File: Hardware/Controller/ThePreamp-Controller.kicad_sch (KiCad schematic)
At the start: 23 parts, among them J1 8V, J2 Power relay trigger, J3 SPI DISPLAY 1, J4 SPI DISPLAY 2, J5 Digital Out, J6 3.3V (Opt), J7 Conn_01x03_Pin, J8 12V, SW1 RotaryEncoder_Switch, SW2 RotaryEncoder_Switch, U1 TSOP34838, U2 CAT24C64WI-GT3, U3 ESP32-DEVKIT-V1, U4 APC-817B1-SL

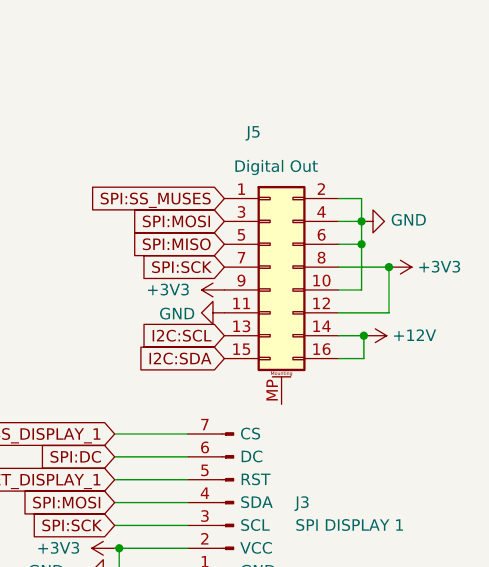
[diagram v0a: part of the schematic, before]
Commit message: Chassis placement new draft
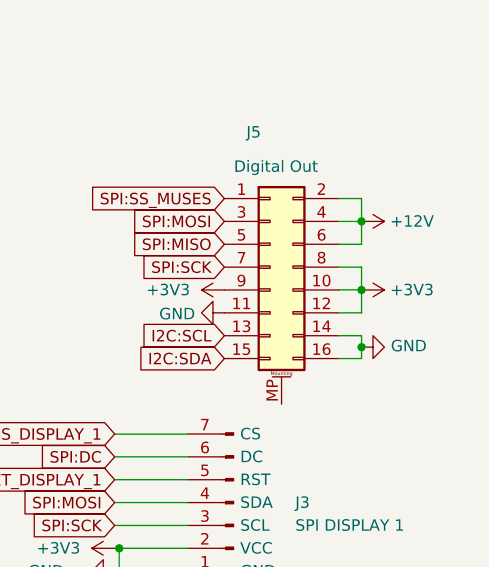
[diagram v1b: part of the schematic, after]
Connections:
- net +12V: now also J5.2 (Pin_2), J5.4 (Pin_4), J5.6 (Pin_6); no longer J5.14 (Pin_14), J5.16 (Pin_16)
- net +3V3: now also J5.10 (Pin_10)
- net GND: now also J5.14 (Pin_14), J5.16 (Pin_16); no longer J5.10 (Pin_10), J5.2 (Pin_2), J5.4 (Pin_4), J5.6 (Pin_6)
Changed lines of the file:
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@@
 	)
 	(junction
-		(at 263.906 62.484)
+		(at 263.906 73.914)
+		(diameter 0)
+		(color 0 0 0 0)
+	)
+	(junction
+		(at 263.906 59.944)
 		(diameter 0)
 		(color 0 0 0 0)
@@
 	)
 	(junction
-		(at 266.954 65.024)
+		(at 263.906 67.564)
 		(diameter 0)
 		(color 0 0 0 0)
@@
 	)
 	(junction
-		(at 264.16 72.644)
-		(diameter 0)
-		(color 0 0 0 0)
-	)
-	(junction
 		(at 117.856 153.67)
 		(diameter 0)
@@
 	)
 	(junction
-		(at 263.906 59.944)
-		(diameter 0)
-		(color 0 0 0 0)
-	)
-	(junction
 		(at 120.396 156.21)
 		(diameter 0)
@@
 	(wire
 		(pts
+			(xy 263.906 65.024) (xy 263.906 67.564)
+		)
+		(stroke
+			(width 0)
+			(type default)
+		)
+	)
+	(wire
+		(pts
+			(xy 263.906 62.484) (xy 263.906 59.944)
+		)
+		(stroke
+			(width 0)
+			(type default)
+		)
+	)
+	(wire
+		(pts
 			(xy 69.596 67.056) (xy 71.882 67.056)
 		)
@@
 	(wire
 		(pts
-			(xy 154.94 66.04) (xy 167.64 66.04)
+			(xy 263.906 57.404) (xy 263.906 59.944)
 		)
 		(stroke
@@
 	(wire
 		(pts
-			(xy 165.1 63.5) (xy 167.64 63.5)
+			(xy 154.94 66.04) (xy 167.64 66.04)
 		)
 		(stroke
@@
 	(wire
 		(pts
-			(xy 124.46 158.75) (xy 117.856 158.75)
+			(xy 165.1 63.5) (xy 167.64 63.5)
 		)
 		(stroke
@@
 	(wire
 		(pts
-			(xy 261.366 72.644) (xy 264.16 72.644)
+			(xy 124.46 158.75) (xy 117.856 158.75)
 		)
 		(stroke
@@
 	(wire
 		(pts
-			(xy 263.906 57.404) (xy 263.906 59.944)
+			(xy 261.366 75.184) (xy 263.906 75.184)
 		)
 		(stroke
@@
 	(wire
 		(pts
-			(xy 263.906 62.484) (xy 263.906 67.564)
+			(xy 263.906 67.564) (xy 263.906 70.104)
 		)
 		(stroke
@@
 	(wire
 		(pts
-			(xy 264.16 75.184) (xy 264.16 72.644)
-		)
-		(stroke
-			(width 0)
-			(type default)
-		)
-	)
-	(wire
-		(pts
 			(xy 236.474 93.726) (xy 244.602 93.726)
 		)
@@
 	(wire
 		(pts
-			(xy 261.366 75.184) (xy 264.16 75.184)
+			(xy 155.702 32.766) (xy 159.766 32.766)
 		)
 		(stroke
@@
 	(wire
 		(pts
-			(xy 155.702 32.766) (xy 159.766 32.766)
+			(xy 236.474 96.266) (xy 236.982 96.266)
 		)
 		(stroke
@@
 	(wire
 		(pts
-			(xy 236.474 96.266) (xy 236.982 96.266)
+			(xy 263.906 72.644) (xy 263.906 73.914)
 		)
 		(stroke
@@
 	(wire
 		(pts
-			(xy 261.366 70.104) (xy 266.954 70.104)
+			(xy 261.366 70.104) (xy 263.906 70.104)
 		)
 		(stroke
@@
 	(wire
 		(pts
-			(xy 263.906 59.944) (xy 263.906 62.484)
+			(xy 125.73 145.542) (xy 125.73 150.114)
 		)
 		(stroke
@@
 	(wire
 		(pts
-			(xy 125.73 145.542) (xy 125.73 150.114)
+			(xy 45.212 100.076) (xy 45.72 100.076)
 		)
 		(stroke
@@
 	(wire
 		(pts
-			(xy 45.212 100.076) (xy 45.72 100.076)
+			(xy 236.728 127.508) (xy 244.856 127.508)
 		)
 		(stroke
@@
 	(wire
 		(pts
-			(xy 236.728 127.508) (xy 244.856 127.508)
+			(xy 261.366 62.484) (xy 263.906 62.484)
 		)
 		(stroke
@@
 	(wire
 		(pts
-			(xy 261.366 62.484) (xy 263.906 62.484)
+			(xy 236.982 107.696) (xy 236.982 118.11)
 		)
 		(stroke
@@
 	(wire
 		(pts
-			(xy 236.982 107.696) (xy 236.982 118.11)
+			(xy 88.9 125.222) (xy 90.17 125.222)
 		)
 		(stroke
@@
 	(wire
 		(pts
-			(xy 88.9 125.222) (xy 90.17 125.222)
+			(xy 77.216 153.67) (xy 77.216 156.21)
 		)
 		(stroke
@@
 	(wire
 		(pts
-			(xy 77.216 153.67) (xy 77.216 156.21)
+			(xy 263.906 73.914) (xy 263.906 75.184)
 		)
 		(stroke
@@
 	(wire
 		(pts
-			(xy 266.954 65.024) (xy 266.954 70.104)
-		)
-		(stroke
-			(width 0)
-			(type default)
-		)
-	)
-	(wire
-		(pts
 			(xy 124.46 156.21) (xy 120.396 156.21)
 		)
@@
 	(wire
 		(pts
-			(xy 261.366 65.024) (xy 266.954 65.024)
+			(xy 261.366 65.024) (xy 263.906 65.024)
 		)
 		(stroke
@@
 	(wire
 		(pts
+			(xy 261.366 72.644) (xy 263.906 72.644)
+		)
+		(stroke
+			(width 0)
+			(type default)
+		)
+	)
+	(wire
+		(pts
 			(xy 86.36 125.222) (xy 86.36 123.952)
 		)
@@
 	(symbol
 		(lib_id "power:+12V")
-		(at 264.16 72.644 270)
+		(at 263.906 59.944 270)
 		(unit 1)
 		(exclude_from_sim no)
@@
 		(fields_autoplaced yes)
 		(property "Reference" "#PWR031"
-			(at 260.35 72.644 0)
+			(at 260.096 59.944 0)
 			(effects
 				(font
@@
 		)
 		(property "Value" "+12V"
-			(at 267.335 72.644 90)
+			(at 267.081 59.944 90)
 			(effects
 				(font
@@
 		)
 		(property "Footprint" ""
-			(at 264.16 72.644 0)
+			(at 263.906 59.944 0)
 			(effects
 				(font
@@
 		)
 		(property "Datasheet" ""
-			(at 264.16 72.644 0)
+			(at 263.906 59.944 0)
 			(effects
 				(font
@@
 		)
 		(property "Description" "Power symbol creates a global label with name \"+12V\""
-			(at 264.16 72.644 0)
+			(at 263.906 59.944 0)
 			(effects
 				(font
@@
 	(symbol
 		(lib_id "power:GND")
-		(at 263.906 59.944 90)
+		(at 263.906 73.914 90)
 		(unit 1)
 		(exclude_from_sim no)
@@
 		(dnp no)
 		(property "Reference" "#PWR023"
-			(at 270.256 59.944 0)
+			(at 270.256 73.914 0)
 			(effects
 				(font
@@
 		)
 		(property "Value" "GND"
-			(at 267.1572 59.817 90)
+			(at 267.1572 73.787 90)
 			(effects
 				(font
@@
 		)
 		(property "Footprint" ""
-			(at 263.906 59.944 0)
+			(at 263.906 73.914 0)
 			(effects
 				(font
@@
 		)
 		(property "Datasheet" ""
-			(at 263.906 59.944 0)
+			(at 263.906 73.914 0)
 			(effects
 				(font
@@
 		)
 		(property "Description" ""
-			(at 263.906 59.944 0)
+			(at 263.906 73.914 0)
 			(effects
 				(font
@@
 	(symbol
 		(lib_id "power:+3.3V")
-		(at 266.954 65.024 270)
+		(at 263.906 67.564 270)
 		(unit 1)
 		(exclude_from_sim no)
@@
 		(fields_autoplaced yes)
 		(property "Reference" "#PWR024"
-			(at 263.144 65.024 0)
+			(at 260.096 67.564 0)
 			(effects
 				(font
@@
 		)
 		(property "Value" "+3V3"
-			(at 270.129 65.024 90)
+			(at 267.081 67.564 90)
 			(effects
 				(font
@@
 		)
 		(property "Footprint" ""
-			(at 266.954 65.024 0)
+			(at 263.906 67.564 0)
 			(effects
 				(font
@@
 		)
 		(property "Datasheet" ""
-			(at 266.954 65.024 0)
+			(at 263.906 67.564 0)
 			(effects
 				(font
@@
 		)
 		(property "Description" ""
-			(at 266.954 65.024 0)
+			(at 263.906 67.564 0)
 			(effects
 				(font
